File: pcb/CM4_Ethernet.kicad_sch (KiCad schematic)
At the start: 14 parts, among them U1 74LVC1G07SE-7, U1 TPD4EUSB30, U2 TPD4EUSB30, U3 MagJack-A70-112-331N126

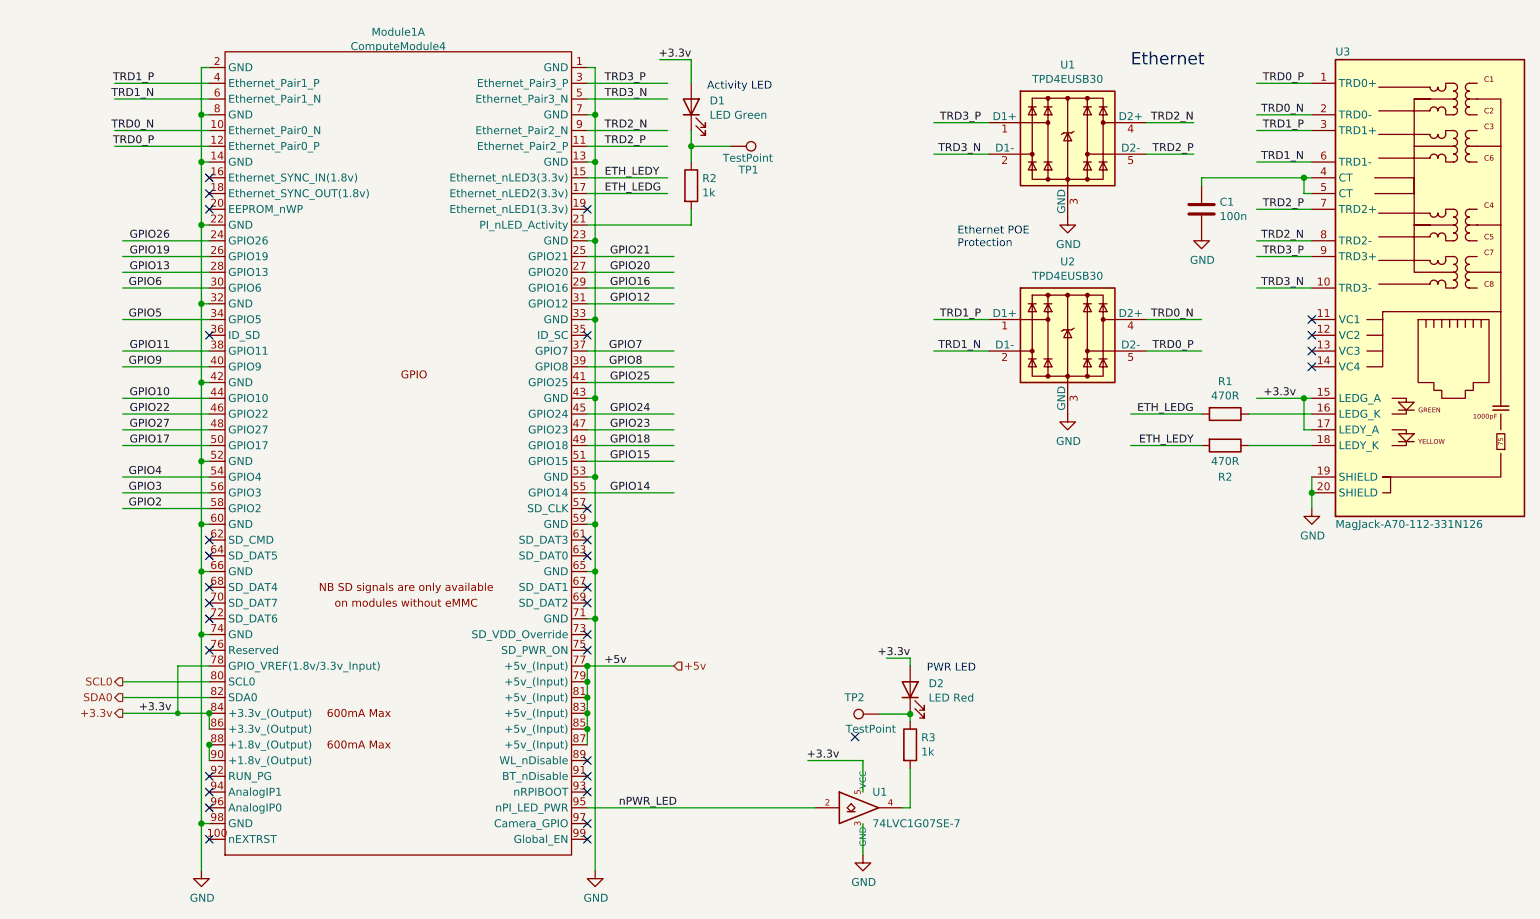
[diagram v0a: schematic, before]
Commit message: - work in progress
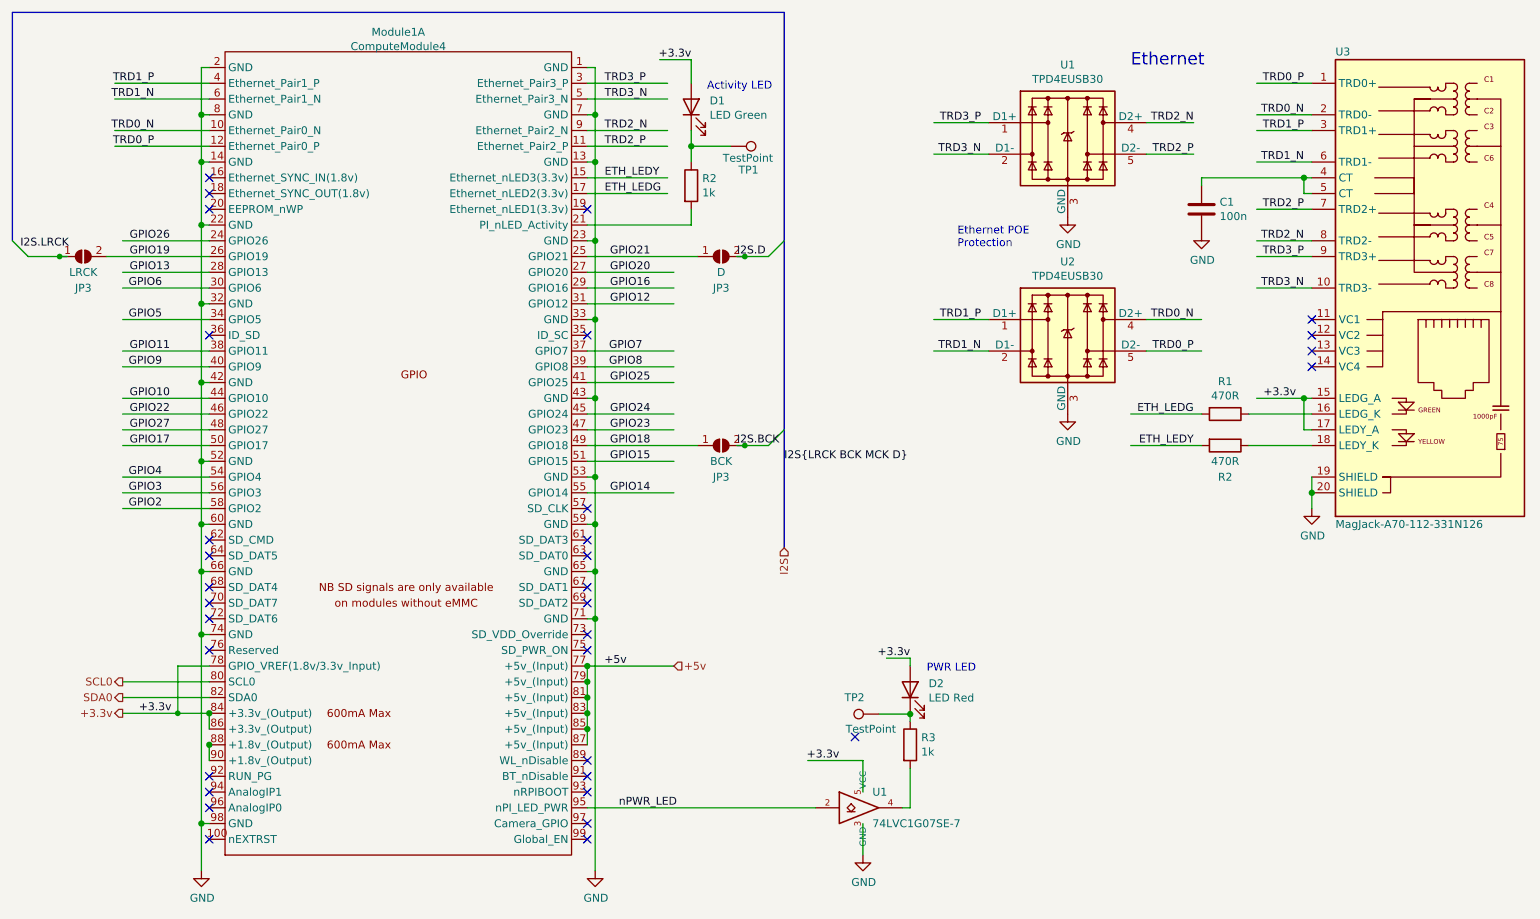
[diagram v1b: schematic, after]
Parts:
- added JP3: LRCK, symbol Jumper:SolderJumper_2_Open
- added JP3: D, symbol Jumper:SolderJumper_2_Open
- added JP3: BCK, symbol Jumper:SolderJumper_2_Open
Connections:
- net GPIO18: now also JP3.1 (A)
- net GPIO19: now also JP3.2 (B)
- net GPIO21: now also JP3.1 (A)
- new net I2S.BCK: JP3.2 (B)
- new net I2S.D: JP3.2 (B)
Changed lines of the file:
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@@
   (junction (at 229.87 97.79) (diameter 1.016) (color 0 0 0 0)
   )
+  (junction (at 138.43 90.17) (diameter 0) (color 0 0 0 0)
+  )
   (junction (at 228.6 46.99) (diameter 1.016) (color 0 0 0 0)
   )
@@
   (junction (at 114.3 95.25) (diameter 1.016) (color 0 0 0 0)
   )
+  (junction (at 138.43 59.69) (diameter 0) (color 0 0 0 0)
+  )
   (junction (at 114.3 57.15) (diameter 1.016) (color 0 0 0 0)
   )
   (junction (at 46.99 133.35) (diameter 0) (color 0 0 0 0)
+  )
+  (junction (at 27.94 59.69) (diameter 0) (color 0 0 0 0)
   )
   (junction (at 114.3 118.11) (diameter 1.016) (color 0 0 0 0)
@@
   (no_connect (at 229.87 72.39))
   (no_connect (at 113.03 72.39))
+  (bus_entry (at 144.78 57.15) (size -2.54 2.54)
+    (stroke (width 0) (type default))
+  )
+  (bus_entry (at 20.32 57.15) (size 2.54 2.54)
+    (stroke (width 0) (type default))
+  )
+  (bus_entry (at 144.78 87.63) (size -2.54 2.54)
+    (stroke (width 0) (type default))
+  )
   (wire (pts (xy 52.07 135.89) (xy 52.07 133.35))
     (stroke (width 0) (type solid))
@@
     (stroke (width 0) (type solid))
   )
+  (wire (pts (xy 29.21 59.69) (xy 27.94 59.69))
+    (stroke (width 0) (type default))
+  )
   (wire (pts (xy 52.07 44.45) (xy 50.8 44.45))
     (stroke (width 0) (type solid))
@@
     (stroke (width 0) (type solid))
   )
+  (bus (pts (xy 144.78 57.15) (xy 144.78 87.63))
+    (stroke (width 0) (type default))
+  )
   (wire (pts (xy 220.98 39.37) (xy 229.87 39.37))
     (stroke (width 0) (type solid))
@@
     (stroke (width 0) (type solid))
   )
+  (wire (pts (xy 138.43 90.17) (xy 142.24 90.17))
+    (stroke (width 0) (type default))
+  )
   (wire (pts (xy 38.1 57.15) (xy 52.07 57.15))
     (stroke (width 0) (type solid))
@@
     (stroke (width 0) (type default))
   )
+  (wire (pts (xy 113.03 59.69) (xy 130.81 59.69))
+    (stroke (width 0) (type solid))
+  )
   (wire (pts (xy 168.91 43.18) (xy 177.8 43.18))
     (stroke (width 0) (type solid))
@@
     (stroke (width 0) (type solid))
   )
+  (bus (pts (xy 20.32 20.32) (xy 20.32 57.15))
+    (stroke (width 0) (type default))
+  )
   (wire (pts (xy 113.03 41.91) (xy 125.984 41.91))
     (stroke (width 0) (type solid))
@@
     (stroke (width 0) (type solid))
   )
+  (wire (pts (xy 35.56 59.69) (xy 52.07 59.69))
+    (stroke (width 0) (type default))
+  )
   (wire (pts (xy 220.98 82.55) (xy 228.6 82.55))
     (stroke (width 0) (type solid))
@@
     (stroke (width 0) (type solid))
   )
+  (bus (pts (xy 144.78 20.32) (xy 144.78 57.15))
+    (stroke (width 0) (type default))
+  )
+  (wire (pts (xy 137.16 90.17) (xy 138.43 90.17))
+    (stroke (width 0) (type default))
+  )
   (wire (pts (xy 38.1 82.55) (xy 52.07 82.55))
     (stroke (width 0) (type solid))
@@
     (stroke (width 0) (type solid))
   )
+  (wire (pts (xy 142.24 59.69) (xy 138.43 59.69))
+    (stroke (width 0) (type default))
+  )
   (wire (pts (xy 38.1 64.77) (xy 52.07 64.77))
     (stroke (width 0) (type solid))
@@
     (stroke (width 0) (type solid))
   )
-  (wire (pts (xy 38.1 59.69) (xy 52.07 59.69))
-    (stroke (width 0) (type solid))
+  (bus (pts (xy 144.78 20.32) (xy 20.32 20.32))
+    (stroke (width 0) (type default))
   )
   (wire (pts (xy 165.1 148.59) (xy 163.83 148.59))
@@
     (stroke (width 0) (type solid))
   )
+  (wire (pts (xy 22.86 59.69) (xy 27.94 59.69))
+    (stroke (width 0) (type default))
+  )
   (wire (pts (xy 113.03 69.85) (xy 114.3 69.85))
     (stroke (width 0) (type solid))
@@
     (stroke (width 0) (type solid))
   )
-  (wire (pts (xy 113.03 90.17) (xy 127 90.17))
-    (stroke (width 0) (type solid))
-  )
   (wire (pts (xy 114.3 95.25) (xy 114.3 102.87))
     (stroke (width 0) (type solid))
@@
     (stroke (width 0) (type solid))
   )
-  (wire (pts (xy 113.03 59.69) (xy 127 59.69))
-    (stroke (width 0) (type solid))
-  )
   (wire (pts (xy 113.03 92.71) (xy 127 92.71))
     (stroke (width 0) (type solid))
@@
     (stroke (width 0) (type solid))
   )
+  (wire (pts (xy 137.16 59.69) (xy 138.43 59.69))
+    (stroke (width 0) (type default))
+  )
   (wire (pts (xy 46.99 133.35) (xy 52.07 133.35))
     (stroke (width 0) (type solid))
@@
     (stroke (width 0) (type solid))
   )
+  (wire (pts (xy 113.03 90.17) (xy 130.81 90.17))
+    (stroke (width 0) (type solid))
+  )
   (wire (pts (xy 220.98 52.07) (xy 229.87 52.07))
     (stroke (width 0) (type solid))
+  )
+  (bus (pts (xy 144.78 87.63) (xy 144.78 106.68))
+    (stroke (width 0) (type default))
   )
   (text "Ethernet" (at 200.66 29.21 0)
@@
     (effects (font (size 1.27 1.27)) (justify right bottom))
   )
+  (label "I2S.BCK" (at 137.16 90.17 0)
+    (effects (font (size 1.27 1.27)) (justify left bottom))
+  )
   (label "GPIO27" (at 45.72 87.63 180) (fields_autoplaced)
     (effects (font (size 1.27 1.27)) (justify right bottom))
@@
   (label "GPIO19" (at 45.72 59.69 180) (fields_autoplaced)
     (effects (font (size 1.27 1.27)) (justify right bottom))
+  )
+  (label "I2S.LRCK" (at 21.59 58.42 0)
+    (effects (font (size 1.27 1.27)) (justify left bottom))
   )
   (label "TRD2_P" (at 115.824 41.91 0) (fields_autoplaced)
@@
     (effects (font (size 1.27 1.27)) (justify left bottom))
   )
+  (label "I2S{LRCK BCK MCK D}" (at 144.78 92.71 0) (fields_autoplaced)
+    (effects (font (size 1.27 1.27)) (justify left bottom))
+  )
   (label "ETH_LEDG" (at 210.82 85.09 180) (fields_autoplaced)
     (effects (font (size 1.27 1.27)) (justify right bottom))
@@
     (effects (font (size 1.27 1.27)) (justify right bottom))
   )
+  (label "I2S.D" (at 137.16 59.69 0)
+    (effects (font (size 1.27 1.27)) (justify left bottom))
+  )
   (label "+3.3v" (at 45.974 133.35 180) (fields_autoplaced)
     (effects (font (size 1.27 1.27)) (justify right bottom))
@@
     (effects (font (size 1.27 1.27)) (justify right))
   )
+  (hierarchical_label "I2S" (shape input) (at 144.78 106.68 270) (fields_autoplaced)
+    (effects (font (size 1.27 1.27)) (justify right))
+  )
   (hierarchical_label "+5v" (shape input) (at 127 125.73 0) (fields_autoplaced)
     (effects (font (size 1.27 1.27)) (justify left))
@@
   (hierarchical_label "SCL0" (shape output) (at 38.1 128.27 180) (fields_autoplaced)
     (effects (font (size 1.27 1.27)) (justify right))
+  )
+  (symbol (lib_id "Jumper:SolderJumper_2_Open") (at 31.75 59.69 0) (unit 1)
+    (in_bom yes) (on_board yes) (dnp no)
+    (property "Reference" "JP3" (at 31.75 64.77 0)
+      (effects (font (size 1.27 1.27)))
+    )
+    (property "Value" "LRCK" (at 31.75 62.23 0)
+      (effects (font (size 1.27 1.27)))
+    )
+    (property "Footprint" "" (at 31.75 59.69 0)
+      (effects (font (size 1.27 1.27)) hide)
+    )
+    (property "Datasheet" "~" (at 31.75 59.69 0)
+      (effects (font (size 1.27 1.27)) hide)
+    )
+    (pin "2")
+    (pin "1")
+    (instances
+      (project "VolumioAmp"
+        (path "/c639bae0-d26f-43ee-9e8c-ca060284bd0b/93301fd2-7a6d-48be-bd24-243a1877e343"
+          (reference "JP3") (unit 1)
+        )
+        (path "/c639bae0-d26f-43ee-9e8c-ca060284bd0b/0d83f7c4-6343-47e0-83de-c41ded3b9d5e"
+          (reference "JP1") (unit 1)
+        )
+      )
+    )
   )
   (symbol (lib_id "CM4IO:TPD4EUSB30") (at 190.5 72.39 0) (unit 1)
@@
         (path "/e63e39d7-6ac0-4ffd-8aa3-1841a4541b55/00000000-0000-0000-0000-00005cff706a"
           (reference "D1") (unit 1)
+        )
+      )
+    )
+  )
+  (symbol (lib_id "Jumper:SolderJumper_2_Open") (at 134.62 59.69 0) (unit 1)
+    (in_bom yes) (on_board yes) (dnp no)
+    (property "Reference" "JP3" (at 134.62 64.77 0)
+      (effects (font (size 1.27 1.27)))
+    )
+    (property "Value" "D" (at 134.62 62.23 0)
+      (effects (font (size 1.27 1.27)))
+    )
+    (property "Footprint" "" (at 134.62 59.69 0)
+      (effects (font (size 1.27 1.27)) hide)
+    )
+    (property "Datasheet" "~" (at 134.62 59.69 0)
+      (effects (font (size 1.27 1.27)) hide)
+    )
+    (pin "2")
+    (pin "1")
+    (instances
+      (project "VolumioAmp"
+        (path "/c639bae0-d26f-43ee-9e8c-ca060284bd0b/93301fd2-7a6d-48be-bd24-243a1877e343"
+          (reference "JP3") (unit 1)
+        )
+        (path "/c639bae0-d26f-43ee-9e8c-ca060284bd0b/0d83f7c4-6343-47e0-83de-c41ded3b9d5e"
+          (reference "JP2") (unit 1)
         )
       )
@@
         )
       )
+    )
+  )
+  (symbol (lib_id "Jumper:SolderJumper_2_Open") (at 134.62 90.17 0) (unit 1)
+    (in_bom yes) (on_board yes) (dnp no)
+    (property "Reference" "JP3" (at 134.62 95.25 0)
+      (effects (font (size 1.27 1.27)))
+    )
+    (property "Value" "BCK" (at 134.62 92.71 0)
+      (effects (font (size 1.27 1.27)))
+    )
+    (property "Footprint" "" (at 134.62 90.17 0)
+      (effects (font (size 1.27 1.27)) hide)
+    )
+    (property "Datasheet" "~" (at 134.62 90.17 0)
+      (effects (font (size 1.27 1.27)) hide)
+    )
+    (pin "2")
+    (pin "1")
+    (instances
+      (project "VolumioAmp"
+        (path "/c639bae0-d26f-43ee-9e8c-ca060284bd0b/93301fd2-7a6d-48be-bd24-243a1877e343"
+          (reference "JP3") (unit 1)
+        )
+        (path "/c639bae0-d26f-43ee-9e8c-ca060284bd0b/0d83f7c4-6343-47e0-83de-c41ded3b9d5e"
+          (reference "JP3") (unit 1)
+        )
+      )
